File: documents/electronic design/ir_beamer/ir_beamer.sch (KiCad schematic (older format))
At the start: 44 parts, among them P1 Via, P10 Via, P11 Via, P12 Via, P13 Via, P14 Via, P15 Via, P16 Via, P17 Via, P18 Via, P19 Via, P2 Via, P20 Via, P21 Via, P3 Via, P4 Via, P5 Via, P6 Via, P7 Via, P8 Via, P9 Via, U1 74HC595D, U2 STM32F103HEADER, U3 74HC595D, U4 SE8R01_module

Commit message: update pcb for beamer
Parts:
- removed P1, P10, P11, P12, P13, P14, P15, P16, P17, P18, P19, P2, P20, P21, P3, P4, P5, P6, P7, P8, P9: Via, footprints:Via, symbol Via
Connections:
- wire segments 36 -> 10

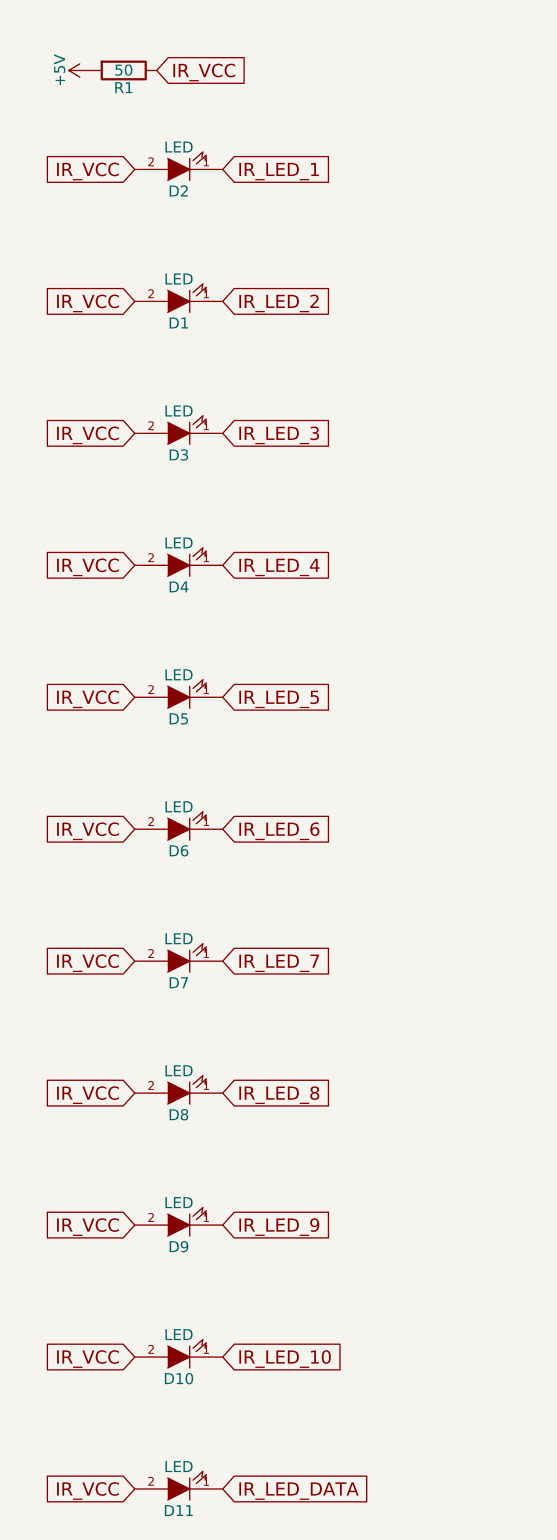
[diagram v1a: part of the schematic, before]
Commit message: fix beamer pcb
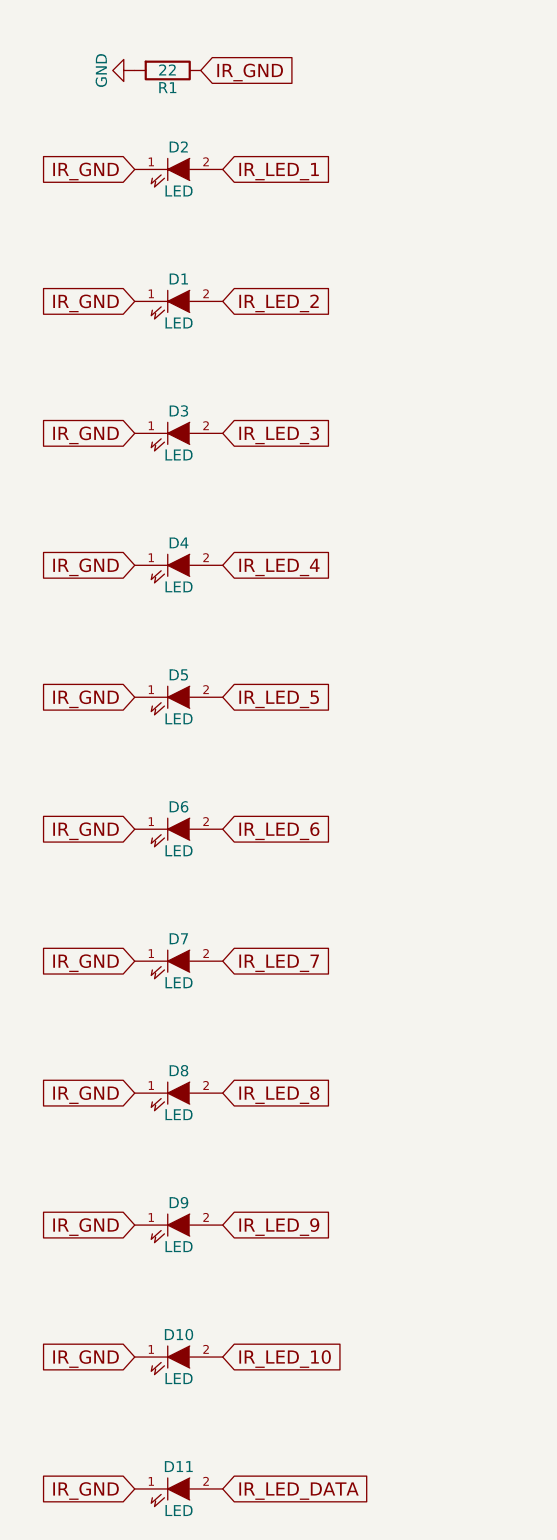
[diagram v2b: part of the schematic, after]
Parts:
- R1: value 50 -> 22
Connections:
- net labels added: IR_GND
- net labels removed: IR_VCC
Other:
- moved on the sheet: R1
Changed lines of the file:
@@
 F 3 "" H 1400 1150 50  0000 C CNN
 	1    1400 1150
-	-1   0    0    1
+	1    0    0    -1
 $EndComp
 Text Notes 8800 1650 0    60   ~ 0
@@
 F 3 "" H 1400 1750 50  0000 C CNN
 	1    1400 1750
-	-1   0    0    1
+	1    0    0    -1
 $EndComp
 Text GLabel 1600 1750 2    60   Input ~ 0
@@
 F 3 "" H 1400 2350 50  0000 C CNN
 	1    1400 2350
-	-1   0    0    1
+	1    0    0    -1
 $EndComp
 Text GLabel 1600 2350 2    60   Input ~ 0
@@
 F 3 "" H 1400 2950 50  0000 C CNN
 	1    1400 2950
-	-1   0    0    1
+	1    0    0    -1
 $EndComp
 Text GLabel 1600 2950 2    60   Input ~ 0
@@
 F 3 "" H 1400 3550 50  0000 C CNN
 	1    1400 3550
-	-1   0    0    1
+	1    0    0    -1
 $EndComp
 Text GLabel 1600 3550 2    60   Input ~ 0
@@
 F 3 "" H 1400 4150 50  0000 C CNN
 	1    1400 4150
-	-1   0    0    1
+	1    0    0    -1
 $EndComp
 Text GLabel 1600 4150 2    60   Input ~ 0
@@
 F 3 "" H 1400 4750 50  0000 C CNN
 	1    1400 4750
-	-1   0    0    1
+	1    0    0    -1
 $EndComp
 Text GLabel 1600 4750 2    60   Input ~ 0
@@
 F 3 "" H 1400 5350 50  0000 C CNN
 	1    1400 5350
-	-1   0    0    1
+	1    0    0    -1
 $EndComp
 Text GLabel 1600 5350 2    60   Input ~ 0
@@
 F 3 "" H 1400 5950 50  0000 C CNN
 	1    1400 5950
-	-1   0    0    1
+	1    0    0    -1
 $EndComp
 Text GLabel 1600 5950 2    60   Input ~ 0
@@
 F 3 "" H 1400 6550 50  0000 C CNN
 	1    1400 6550
-	-1   0    0    1
+	1    0    0    -1
 $EndComp
 Text GLabel 1600 6550 2    60   Input ~ 0
@@
 F 3 "" H 1400 7150 50  0000 C CNN
 	1    1400 7150
-	-1   0    0    1
+	1    0    0    -1
 $EndComp
 Text GLabel 4700 2700 2    60   Input ~ 0
@@
 	1    0    0    -1
 $EndComp
-$Comp
-L +5V #PWR012
-U 1 1 5791C22D
-P 1000 700
-F 0 "#PWR012" H 1000 550 50  0001 C CNN
-F 1 "+5V" H 1000 840 50  0000 C CNN
-F 2 "" H 1000 700 50  0000 C CNN
-F 3 "" H 1000 700 50  0000 C CNN
-	1    1000 700
-	0    -1   -1   0
-$EndComp
 Text GLabel 4700 1350 2    60   Input ~ 0
 Cascade
@@
 L R R1
 U 1 1 57A138ED
-P 1150 700
-F 0 "R1" V 1230 700 50  0000 C CNN
-F 1 "50" V 1150 700 50  0000 C CNN
-F 2 "Capacitors_SMD:C_0805_HandSoldering" V 1080 700 50  0001 C CNN
-F 3 "" H 1150 700 50  0000 C CNN
-	1    1150 700
-	0    1    1    0
-$EndComp
-Text GLabel 1300 700  2    60   Input ~ 0
-IR_VCC
-Text GLabel 1200 1150 0    60   Input ~ 0
-IR_VCC
-Text GLabel 1200 1750 0    60   Input ~ 0
-IR_VCC
-Text GLabel 1200 2350 0    60   Input ~ 0
-IR_VCC
-Text GLabel 1200 2950 0    60   Input ~ 0
-IR_VCC
-Text GLabel 1200 3550 0    60   Input ~ 0
-IR_VCC
-Text GLabel 1200 4150 0    60   Input ~ 0
-IR_VCC
-Text GLabel 1200 4750 0    60   Input ~ 0
-IR_VCC
-Text GLabel 1200 5350 0    60   Input ~ 0
-IR_VCC
-Text GLabel 1200 5950 0    60   Input ~ 0
-IR_VCC
-Text GLabel 1200 6550 0    60   Input ~ 0
-IR_VCC
-Text GLabel 1200 7150 0    60   Input ~ 0
-IR_VCC
+P 1350 700
+F 0 "R1" V 1430 700 50  0000 C CNN
+F 1 "22" V 1350 700 50  0000 C CNN
+F 2 "Capacitors_SMD:C_0805_HandSoldering" V 1280 700 50  0001 C CNN
+F 3 "" H 1350 700 50  0000 C CNN
+	1    1350 700
+	0    1    1    0
+$EndComp
+Text GLabel 1500 700  2    60   Input ~ 0
+IR_GND
 Text GLabel 3800 3000 0    60   Input ~ 0
 IR_LED_DATA
@@
 	5200 2900 4700 2900
 NoConn ~ 3800 750
+$Comp
+L GND #PWR?
+U 1 1 57AB0120
+P 1200 700
+F 0 "#PWR?" H 1200 450 50  0001 C CNN
+F 1 "GND" H 1200 550 50  0000 C CNN
+F 2 "" H 1200 700 50  0000 C CNN
+F 3 "" H 1200 700 50  0000 C CNN
+	1    1200 700
+	0    1    1    0
+$EndComp
+Text GLabel 1200 1150 0    60   Input ~ 0
+IR_GND
+Text GLabel 1200 1750 0    60   Input ~ 0
+IR_GND
+Text GLabel 1200 2350 0    60   Input ~ 0
+IR_GND
+Text GLabel 1200 2950 0    60   Input ~ 0
+IR_GND
+Text GLabel 1200 3550 0    60   Input ~ 0
+IR_GND
+Text GLabel 1200 4150 0    60   Input ~ 0
+IR_GND
+Text GLabel 1200 4750 0    60   Input ~ 0
+IR_GND
+Text GLabel 1200 5350 0    60   Input ~ 0
+IR_GND
+Text GLabel 1200 5950 0    60   Input ~ 0
+IR_GND
+Text GLabel 1200 6550 0    60   Input ~ 0
+IR_GND
+Text GLabel 1200 7150 0    60   Input ~ 0
+IR_GND
 $EndSCHEMATC
